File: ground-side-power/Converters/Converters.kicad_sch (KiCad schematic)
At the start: 43 parts, among them J10 Conn_01x03_Female, J11 Ground Connections, J12 Conn_01x04_Female, J13 DAQ Voltage Sensing, J14 DAQ Current Sensing, J27 Conn_01x02_Female, U1 TPS55340, U2 K7805-3AR3, U4 INA180, U5 INA180

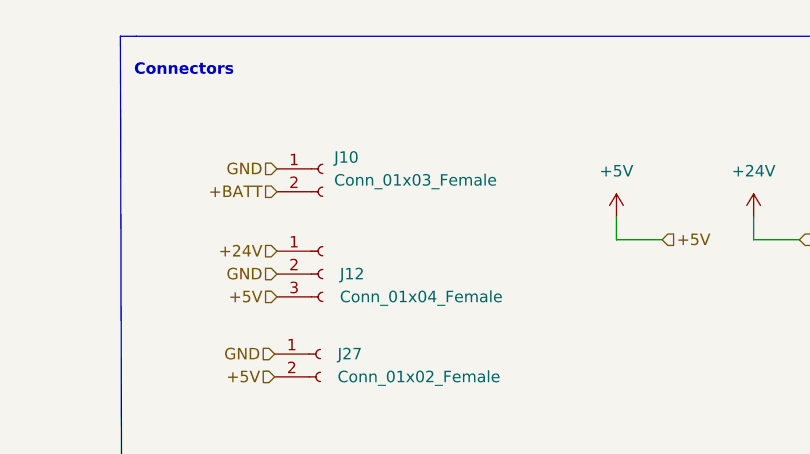
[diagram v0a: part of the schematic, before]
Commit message: Created layout
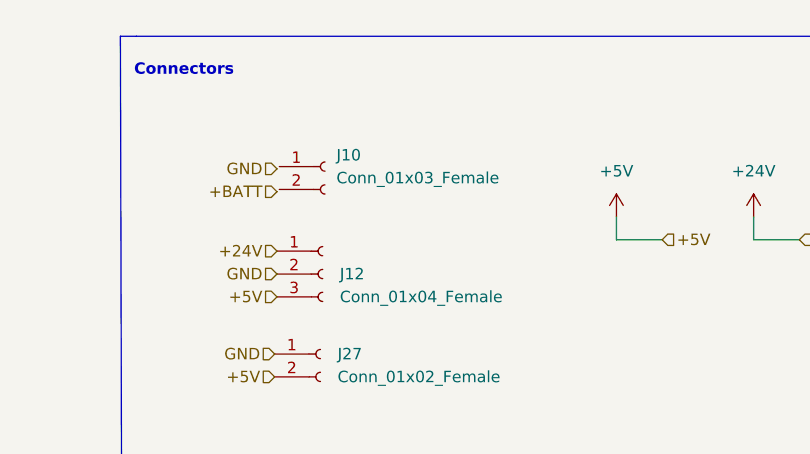
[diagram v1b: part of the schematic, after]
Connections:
- net +BATT: no longer J10.2 (Pin_2)
- net GND: no longer J10.1 (Pin_1)
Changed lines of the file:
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@@
     )
   )
-  (symbol (lib_id "Connector:Conn_01x02_Female") (at 185.166 32.004 0) (unit 1)
+  (symbol (lib_id "Connector:Conn_01x02_Female") (at 185.42 31.75 0) (unit 1)
     (in_bom yes) (on_board yes) (dnp no) (fields_autoplaced)
-    (property "Reference" "J10" (at 186.436 30.7339 0)
+    (property "Reference" "J10" (at 186.69 30.4799 0)
       (effects (font (size 1.27 1.27)) (justify left))
     )
-    (property "Value" "Conn_01x03_Female" (at 186.436 33.2739 0)
+    (property "Value" "Conn_01x03_Female" (at 186.69 33.0199 0)
       (effects (font (size 1.27 1.27)) (justify left))
     )
-    (property "Footprint" "GSP:1935310" (at 185.166 32.004 0)
+    (property "Footprint" "GSP:1935310" (at 185.42 31.75 0)
       (effects (font (size 1.27 1.27)) hide)
     )
-    (property "Datasheet" "~" (at 185.166 32.004 0)
+    (property "Datasheet" "~" (at 185.42 31.75 0)
       (effects (font (size 1.27 1.27)) hide)
     )
